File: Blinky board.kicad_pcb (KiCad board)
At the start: 2 copper layers, 104.4 x 84.2 mm, 23 parts, among them SW1 SW_Push, U1 ICM7555xB

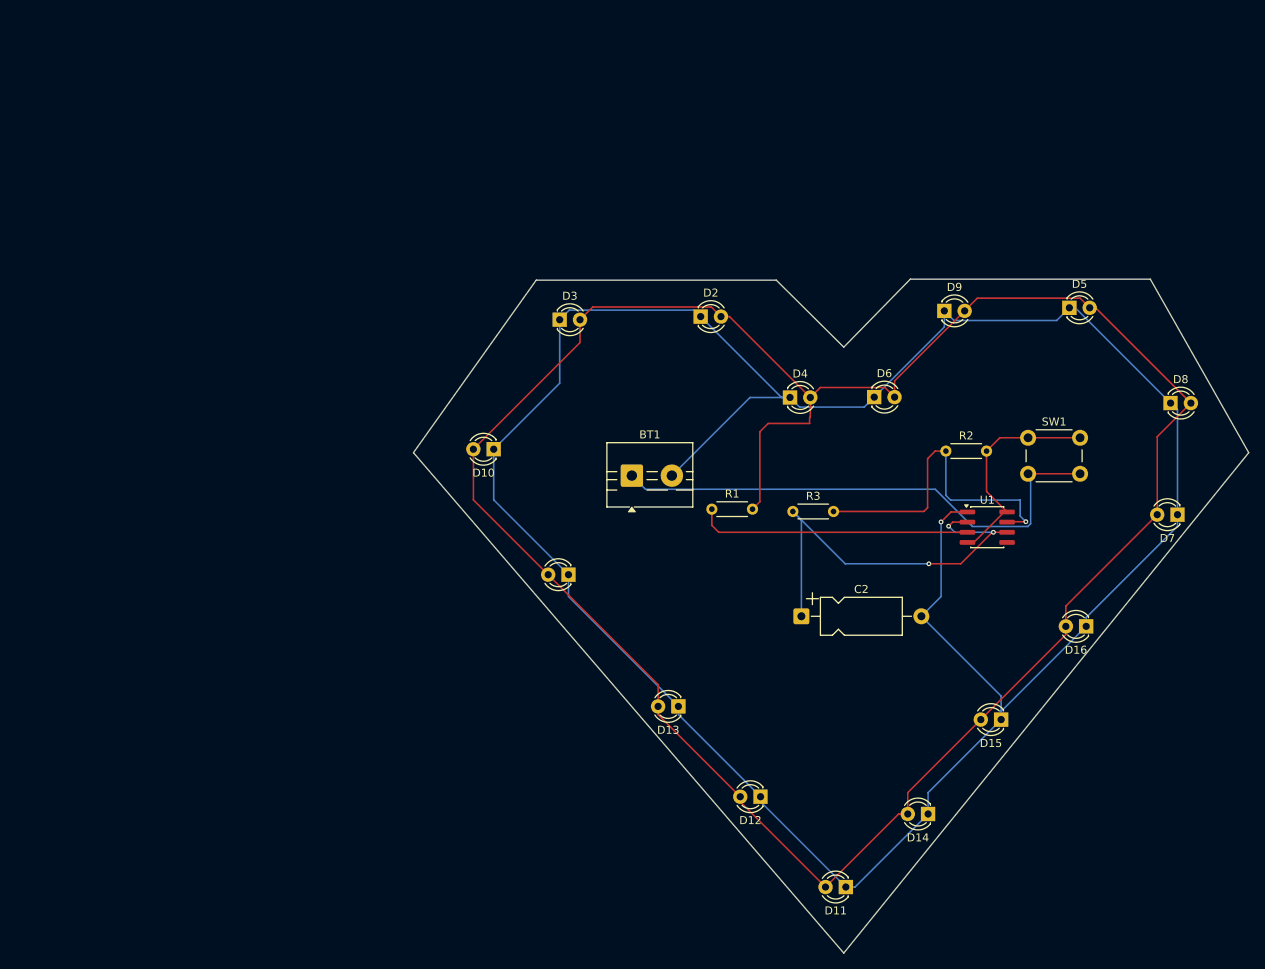
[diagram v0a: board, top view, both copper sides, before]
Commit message: Add files via upload
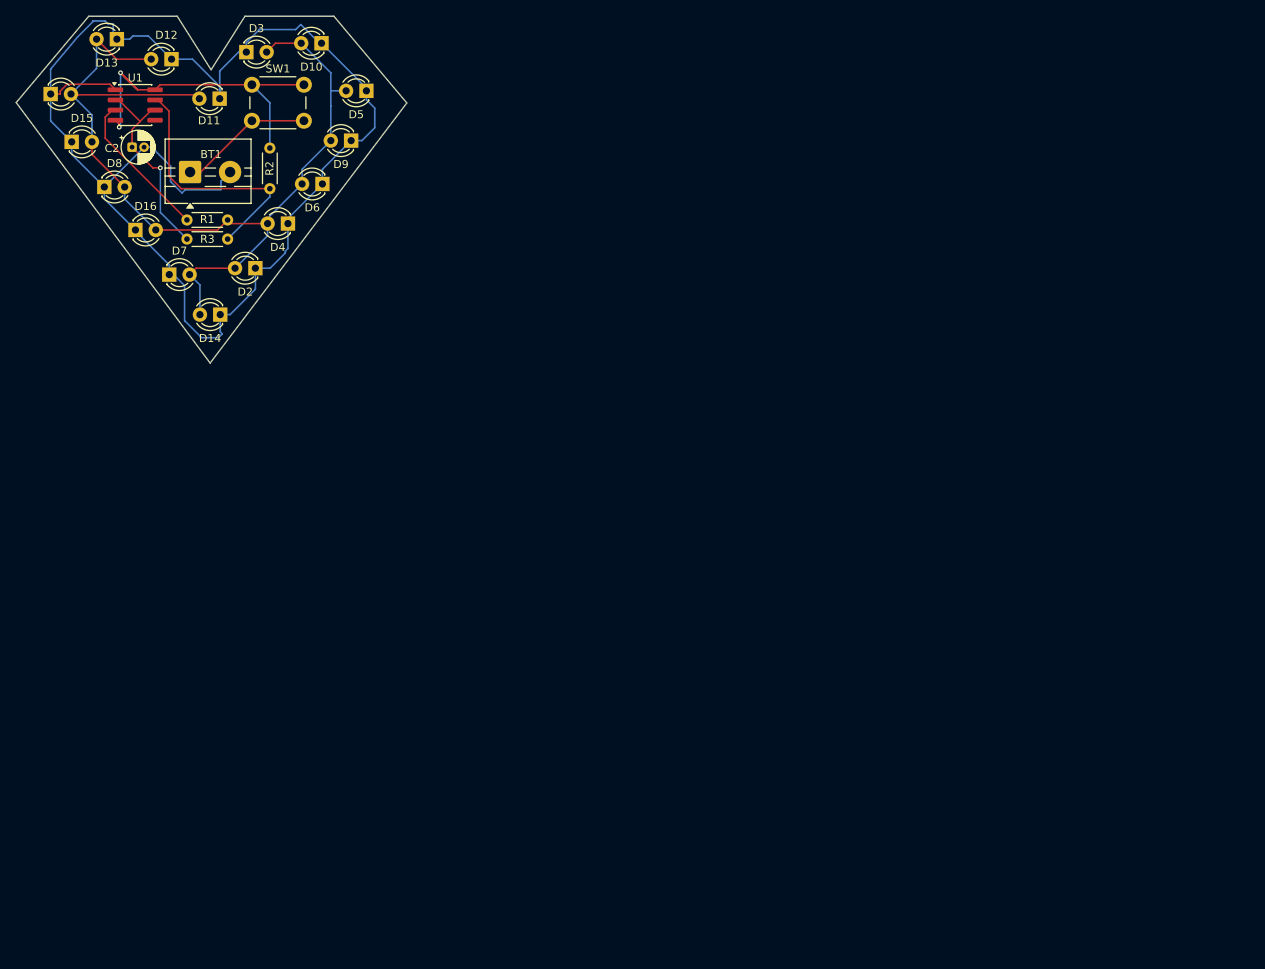
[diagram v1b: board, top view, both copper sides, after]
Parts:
- C2: footprint Capacitor_THT:CP_Axial_L10.0mm_D4.5mm_P15.00mm_Horizontal -> Capacitor_THT:CP_Radial_D4.0mm_P1.50mm
- moved D15 136.8 mm to (48.9, 60.2), turned to 0 degrees
- moved D8 136.0 mm to (53.0, 65.9)
- moved D7 129.6 mm to (61.1, 76.8), turned to 0 degrees
- moved D16 128.8 mm to (56.9, 71.2), turned to 0 degrees
- moved D11 125.8 mm to (67.4, 54.8)
- moved U1 118.9 mm to (56.9, 55.6)
- moved D12 118.0 mm to (61.4, 49.9)
- moved D13 109.0 mm to (54.6, 47.4)
- moved D14 108.3 mm to (67.5, 81.8)
- moved SW1 106.6 mm to (71.5, 53.1)
- moved C2 102.2 mm to (56.5, 60.9)
- moved D5 92.0 mm to (85.8, 53.9), turned to 180 degrees
- moved R2 90.6 mm to (73.7, 66.1), turned to 90 degrees
- moved D1 88.3 mm to (46.3, 54.3), turned to 0 degrees
- moved R3 83.0 mm to (63.3, 72.4)
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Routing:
- net TOUT: track 289.2 -> 121.3 mm
- net GND: track 317.9 -> 176.7 mm, vias 1 -> 0
- net Net-(BT1-+): track 65.5 -> 16.9 mm
- net Net-(U1-THRES): track 53.1 -> 25.2 mm, vias 3 -> 1
- net Net-(U1-VCC): track 27.6 -> 53.0 mm, vias 0 -> 2
- net Net-(U1-OUT): track 34.3 -> 18.7 mm
- net Net-(U1-DISCH): track 41.2 -> 32.2 mm, vias 1 -> 0
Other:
- board size 104.4 x 84.2 mm -> 48.8 x 43.4 mm
